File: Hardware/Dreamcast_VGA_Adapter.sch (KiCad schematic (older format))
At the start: 44 parts, among them J1 AudioJack3, J2 DB15_Female_HighDensity_Mount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, J3 Conn_02x08_Odd_Even, SW1 SW_DIP_x02, U1 THS7316, U2 74HCT2G34

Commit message: Update Dreamcast_VGA_Adapter.sch
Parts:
- C21: Manufacturer Part Number (none) -> CC0805MKX7R7BB105
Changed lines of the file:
@@
 F 2 "Capacitor_SMD:C_0805_2012Metric_Pad1.15x1.40mm_HandSolder" H 2638 6250 50  0001 C CNN
 F 3 "~" H 2600 6400 50  0001 C CNN
-F 4 "" H 2600 6400 50  0001 C CNN "Manufacturer Part Number"
+F 4 "CC0805MKX7R7BB105" H 2600 6400 50  0001 C CNN "Manufacturer Part Number"
 	1    2600 6400
 	1    0    0    -1

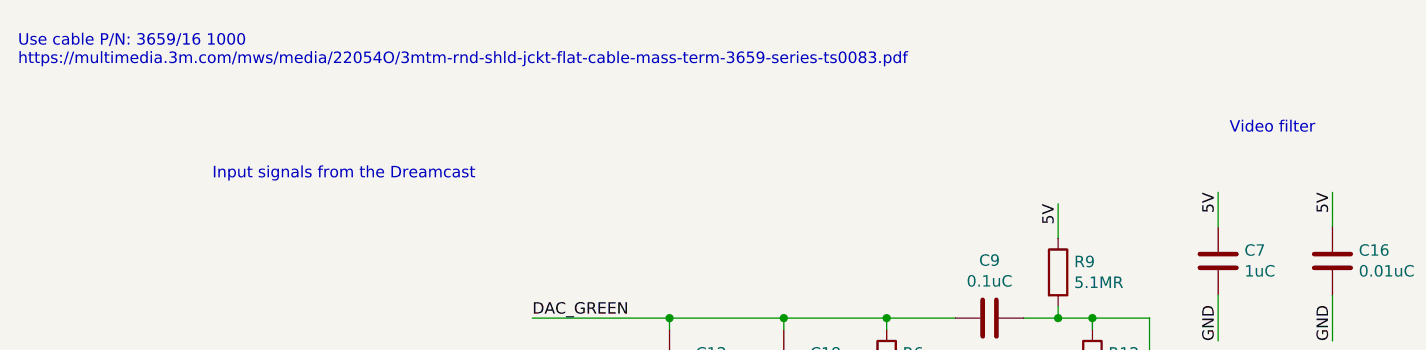
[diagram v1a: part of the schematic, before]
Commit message: Progressed circuit design.
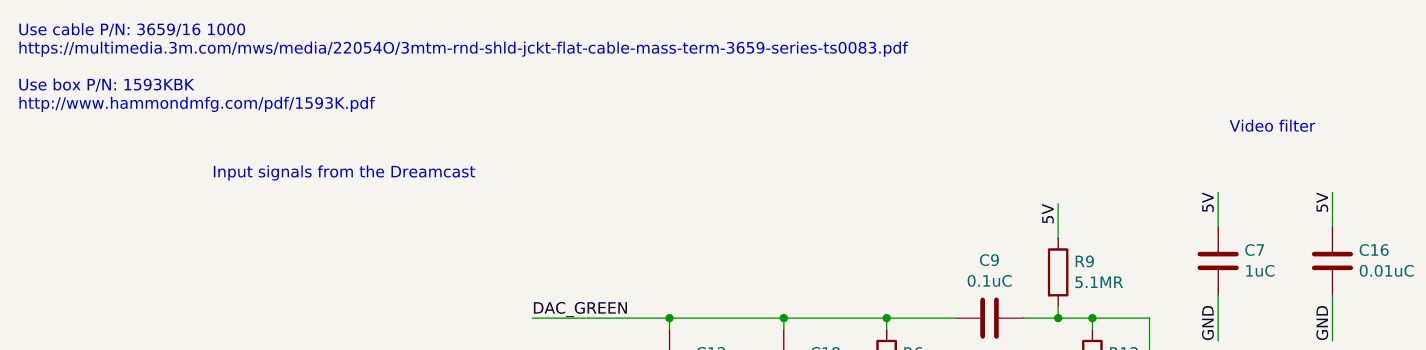
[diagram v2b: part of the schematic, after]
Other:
- note added: "Use cable P/N: 3659/16 1000\nhttps://multimedia.3m.com/mws/media/22054O/3mtm-rnd-shld-jckt-flat-cable-mass-term-3659-series-ts0083.pdf\n\nUse box P/N: 1593KBK\nhttp://www.hammondmfg.com/pdf/1593K.pdf"
- note removed: "Use cable P/N: 3659/16 1000\nhttps://multimedia.3m.com/mws/media/22054O/3mtm-rnd-shld-jckt-flat-cable-mass-term-3659-series-ts0083.pdf"
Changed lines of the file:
@@
 	1    0    0    -1
 $EndComp
-Text Notes 550  700  0    50   ~ 0
-Use cable P/N: 3659/16 1000\nhttps://multimedia.3m.com/mws/media/22054O/3mtm-rnd-shld-jckt-flat-cable-mass-term-3659-series-ts0083.pdf
+Text Notes 550  900  0    50   ~ 0
+Use cable P/N: 3659/16 1000\nhttps://multimedia.3m.com/mws/media/22054O/3mtm-rnd-shld-jckt-flat-cable-mass-term-3659-series-ts0083.pdf\n\nUse box P/N: 1593KBK\nhttp://www.hammondmfg.com/pdf/1593K.pdf
 Wire Wire Line
 	1250 6150 1050 6150

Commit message: Progressed circuit design.
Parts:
- J3: footprint (none) -> Connector_IDC:IDC-Header_2x08_P2.54mm_Vertical
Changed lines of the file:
@@
 F 0 "J3" H 1550 3367 50  0000 C CNN
 F 1 "Conn_02x08_Odd_Even" H 1550 3276 50  0000 C CNN
-F 2 "" H 1500 2850 50  0001 C CNN
+F 2 "Connector_IDC:IDC-Header_2x08_P2.54mm_Vertical" H 1500 2850 50  0001 C CNN
 F 3 "https://multimedia.3m.com/mws/media/375264O/3mtm-100-in-pcb-100x-100-two-row-78xx-series-ts2104.pdf" H 1500 2850 50  0001 C CNN
 F 4 "7816-0000PR" H 1500 2850 50  0001 C CNN "Manufacturer Part Number"
